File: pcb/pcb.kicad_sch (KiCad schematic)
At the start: 27 parts, among them J1 Conn_02x08_Top_Bottom, SW1 CherryMX_LED, SW2 CherryMX_LED, SW3 1241.1100.7095, SW4 SW_SPST, U1 ICM7211AMIPL, U2 ICM7211AMIPL, U3 ATTINY44A, U4 NL37WZ14USG, U5 CD74ACT139E, U6 MAX5035BUSA+, Y1 Crystal

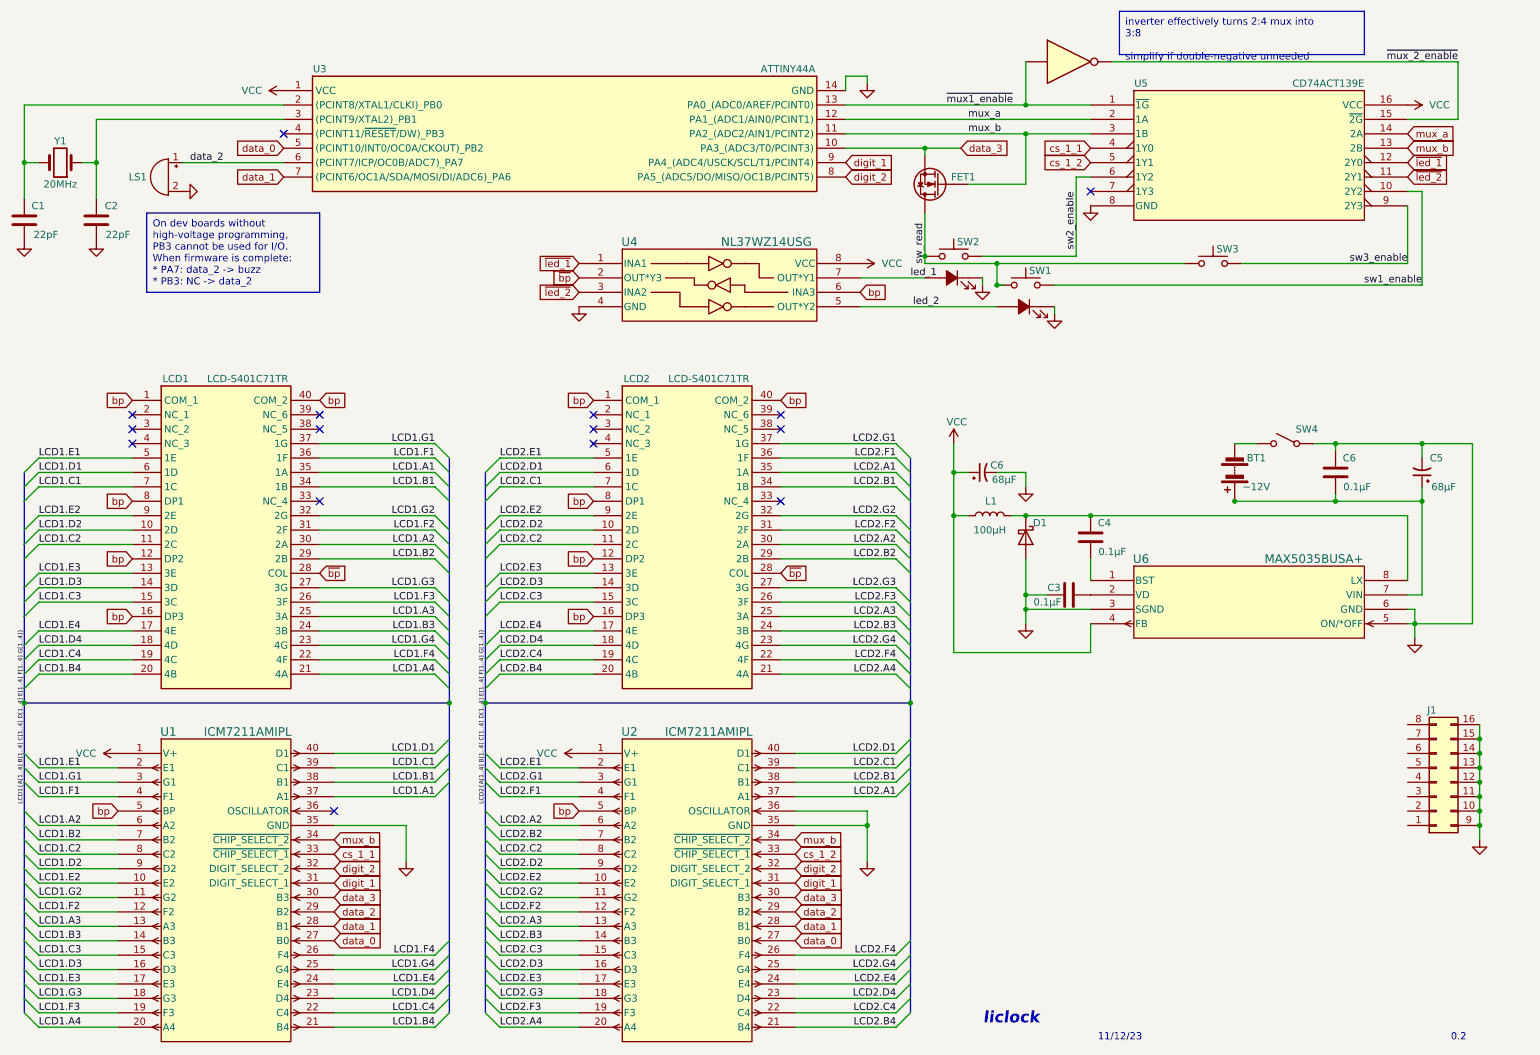
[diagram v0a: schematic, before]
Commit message: Update schematic
Signed-off-by: Michael Darr <michael.e.darr@gmail.com>
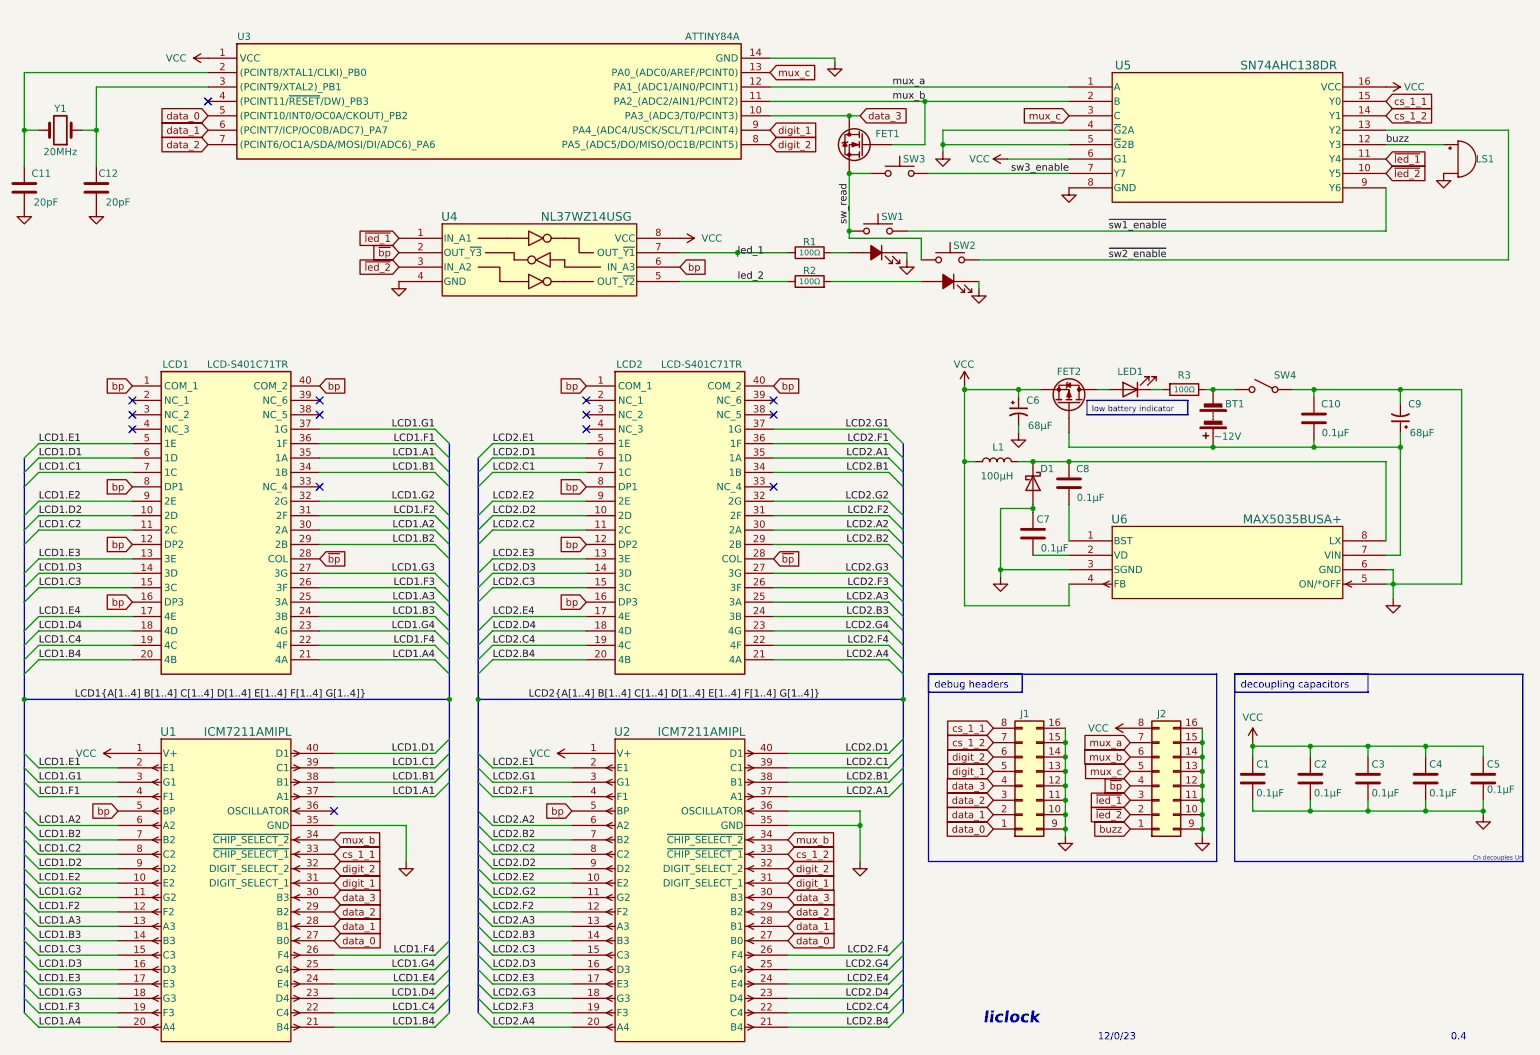
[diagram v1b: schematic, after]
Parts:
- removed U5: CD74ACT139E, N16, symbol Clock-Parts:CD74ACT139E
- removed U?: 74AHC04, symbol 74xx:74AHC04
- added C1, C2, C3, C4, C5: 0.1µF, symbol Device:C
- added FET2: XP9561GI, symbol Simulation_SPICE:PMOS
- added J2: Conn_02x08_Top_Bottom, symbol Connector_Generic:Conn_02x08_Top_Bottom
- added LED1: 151033RS03000, symbol Device:LED
- added R1, R2, R3: 100Ω, symbol Device:R
- added U5: SN74AHC138DR, D16, symbol Clock-Parts:SN74AHC138DR
- C11: renamed from C1; Capacitance 22pF -> 20pF
- C12: renamed from C2; Capacitance 22pF -> 20pF
- FET1: PN (none) -> 2N7002-G
- U3: value ATTINY44A -> ATTINY84A; Arrow Part Number ATTINY44A-PU -> (none); Arrow Price/Stock https://www.arrow.com/en/products/attiny44a-pu/microchip-te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 -> (none); Manufacturer_Part_Number ATTINY44A-PU -> ATTINY48A-PU; Mouser Part Number 556-ATTINY44A-PU -> (none); Mouser Price/Stock https://www.mouser.co.uk/ProductDetail/Microchip-Technology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 -> (none)
- renumbered C6 to C10, C3 to C7, C4 to C8, C5 to C9, SW2 to SW1, SW1 to SW2
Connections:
- net GND: now also C7.1, C1.2, C2.2, C3.2, C4.2, C5.2, J2.10 (Pin_10), J2.11 (Pin_11), J2.12 (Pin_12), J2.13 (Pin_13), J2.14 (Pin_14), J2.15 (Pin_15), J2.16 (Pin_16), J2.9 (Pin_9), U5.4 (~{G}2A), U5.5 (~{G}2B), U5.8 (GND); no longer C7.2
- net VCC: now also C1.1, C2.1, C3.1, C4.1, C5.1, FET2.3 (S), J2.8 (Pin_8), U5.16 (VCC), U5.6 (G1)
- net cs_1_1: now also J1.8 (Pin_8), U5.15 (Y0)
- net cs_1_2: now also J1.7 (Pin_7), U5.14 (Y1)
- net data_0: now also J1.1 (Pin_1)
- net data_1: now also J1.2 (Pin_2), U3.6 ((PCINT7/ICP/OC0B/ADC7)_PA7); no longer U3.7 ((PCINT6/OC1A/SDA/MOSI/DI/ADC6)_PA6)
- net data_2: now also J1.3 (Pin_3), U3.7 ((PCINT6/OC1A/SDA/MOSI/DI/ADC6)_PA6); no longer LS1.1 (-), U3.6 ((PCINT7/ICP/OC0B/ADC7)_PA7)
- net data_3: now also FET1.2 (D), J1.4 (Pin_4); no longer FET1.3 (S)
- net digit_1: now also J1.5 (Pin_5)
- net digit_2: now also J1.6 (Pin_6)
- net led_1: now also R1.1; no longer SW1.4 (A)
- net led_2: now also R2.1; no longer SW2.4 (A)
- net mux_a: now also J2.7 (Pin_7), U5.1 (A)
- net mux_b: now also J2.6 (Pin_6), U5.2 (B)
- net sw3_enable: now also U5.7 (Y7)
- net sw_read: now also FET1.3 (S); no longer FET1.2 (D)
- net ~{bp}: now also J2.4 (Pin_4)
- net ~{led_1}: now also J2.3 (Pin_3), U5.11 (Y4)
- net ~{led_2}: now also J2.2 (Pin_2), U5.10 (Y5)
- net at BT1.1 (+), C10.2, C9.1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: now also FET2.2 (G)
- net at BT1.2 (-), SW4.2 (B): now also R3.1
- net at U6.2 (VD): now also C7.2; no longer C7.1
- net sw1_enable renamed ~{sw2_enable}
- net ~{sw2_enable}: now also U5.13 (Y2)
- net sw2_enable renamed ~{sw1_enable}
- net ~{sw1_enable}: now also U5.9 (Y6)
- net ~{mux1_enable} renamed mux_c
- net mux_c: now also J2.5 (Pin_5), U5.3 (C)
- new net: LED1.1 (K), R3.2
- new net: R1.2, SW1.4 (A)
- new net: FET2.1 (D), LED1.2 (A)
- new net: R2.2, SW2.4 (A)
- new net buzz: J2.1 (Pin_1), LS1.1 (-), U5.12 (Y3)
- no-connect marks 15 -> 14
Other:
- note added: "0.4"
- note added: "12/0/23"
- note added: "Cn decouples Un"
- note removed: "0.2"
- note removed: "11/12/23"
- moved on the sheet: BT1, C10, C11, C12, C6, C7, C8, C9, D1, FET1, J1, L1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
